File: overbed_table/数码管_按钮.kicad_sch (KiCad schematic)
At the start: 29 parts, among them SW1 KH-6X6X6H-STM, SW10 KH-6X6X6H-STM, SW11 KH-6X6X6H-STM, SW12 KH-6X6X6H-STM, SW2 KH-6X6X6H-STM, SW3 KH-6X6X6H-STM, SW4 KH-6X6X6H-STM, SW5 KH-6X6X6H-STM, SW6 KH-6X6X6H-STM, SW7 KH-6X6X6H-STM, SW8 KH-6X6X6H-STM, SW9 KH-6X6X6H-STM, U3 TM1638

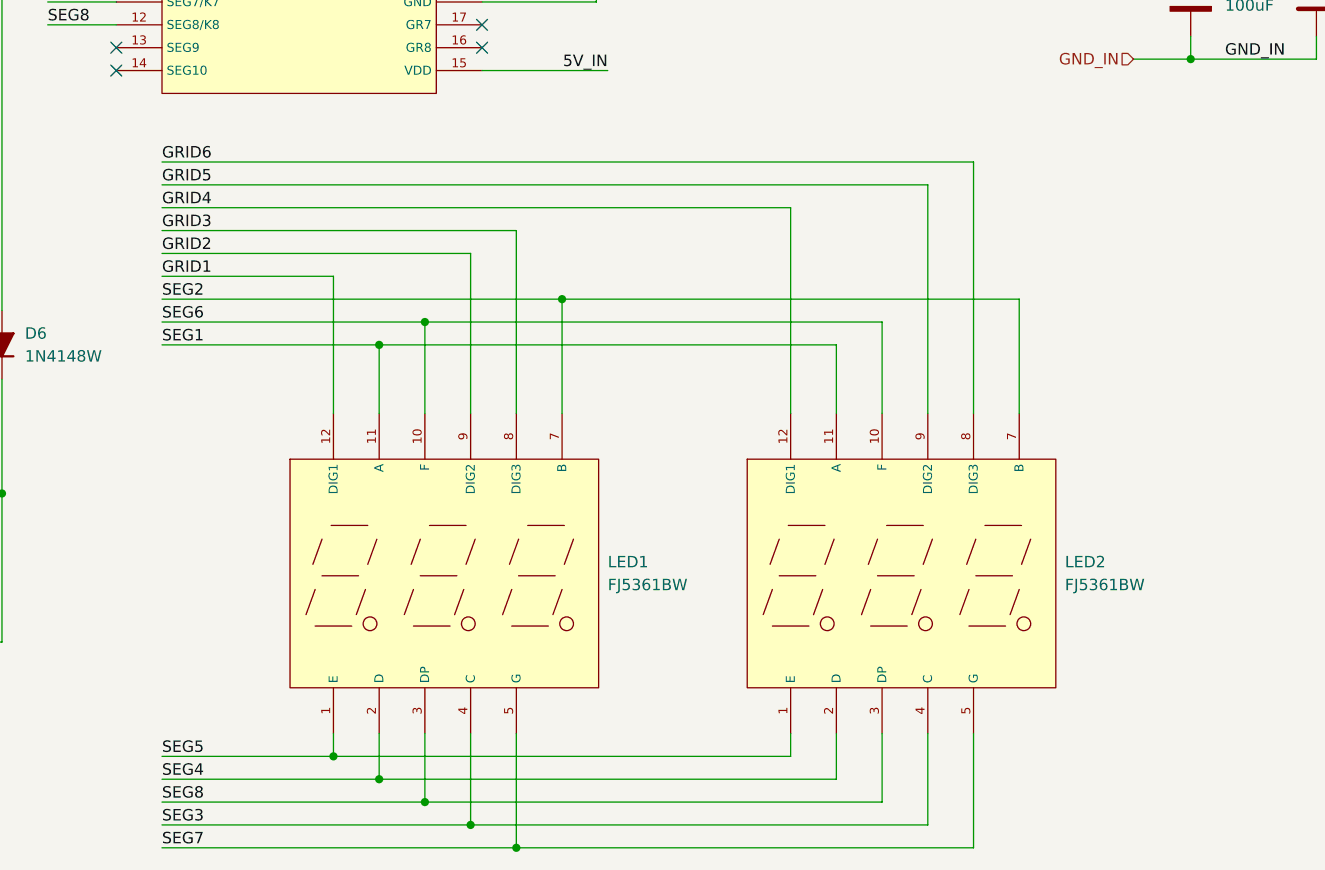
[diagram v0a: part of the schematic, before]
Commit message: 更新原理图
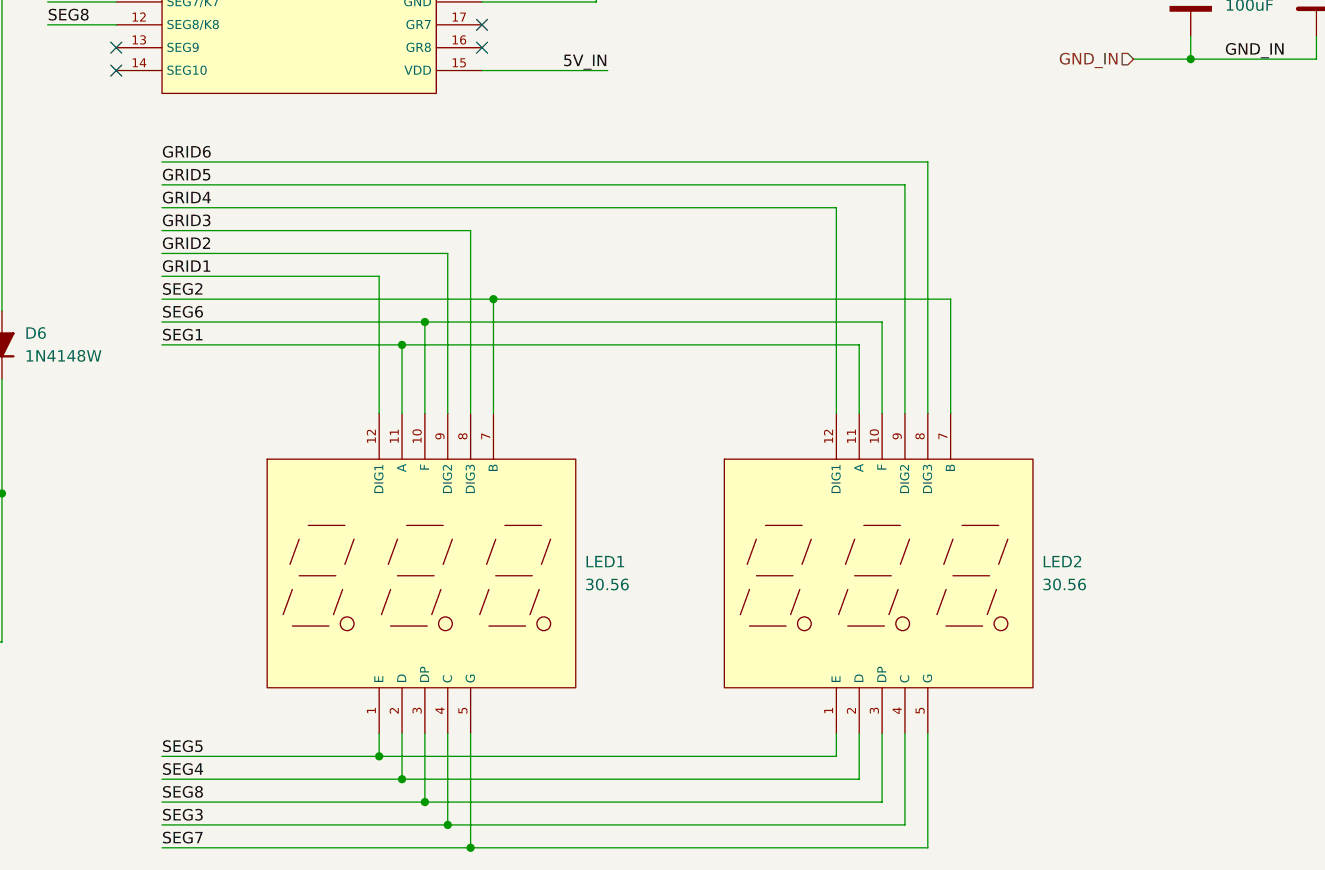
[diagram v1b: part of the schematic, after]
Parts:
- removed LED1, LED2: FJ5361BW, lcsc_footprints:C2938342_LED-SEG-TH_11P-L37_5-W19_0-P2_54-LS15_2-BL, symbol lcsc_imported:FJ5361BW
- added LED1, LED2: 30.56, lcsc_footprints:C18187_LED-SEG-TH_FJ5361AH, symbol lcsc_imported:30_56
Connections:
- net GRID1: now also LED1.12 (DIG1)
- net GRID2: now also LED1.9 (DIG2)
- net GRID3: now also LED1.8 (DIG3)
- net GRID4: now also LED2.12 (DIG1)
- net GRID5: now also LED2.9 (DIG2)
- net GRID6: now also LED2.8 (DIG3)
- net SEG1: now also LED1.11 (A), LED2.11 (A)
- net SEG2: now also LED1.7 (B), LED2.7 (B)
- net SEG3: now also LED1.4 (C), LED2.4 (C)
- net SEG4: now also LED1.2 (D), LED2.2 (D)
- net SEG5: now also LED1.1 (E), LED2.1 (E)
- net SEG6: now also LED1.10 (F), LED2.10 (F)
- net SEG7: now also LED1.5 (G), LED2.5 (G)
- net SEG8: now also LED1.3 (DP), LED2.3 (DP)
